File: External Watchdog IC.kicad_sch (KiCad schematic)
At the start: 10 parts, among them U4 TPS3823A-33DBVR, U5 TPS3823A-33DBVR

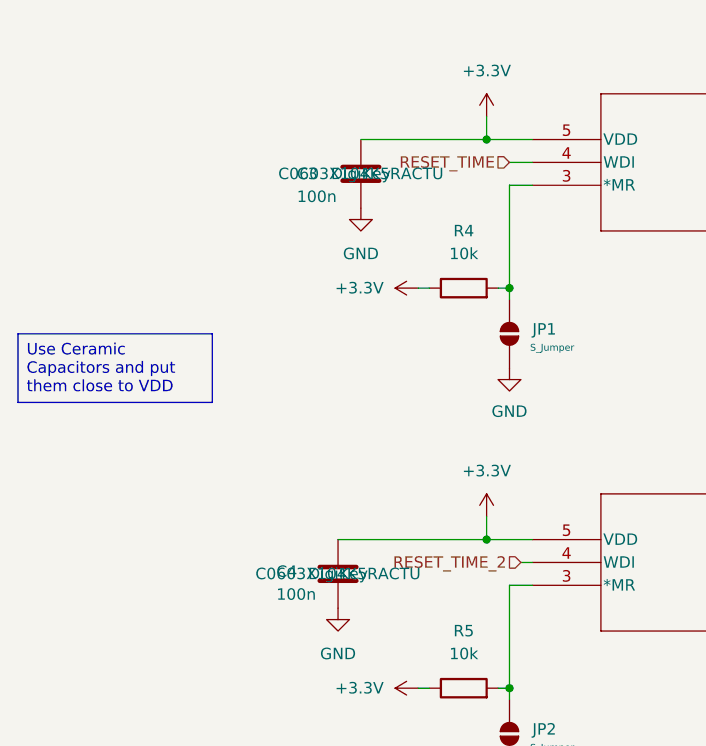
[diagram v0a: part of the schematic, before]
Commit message: Added footprints to caps
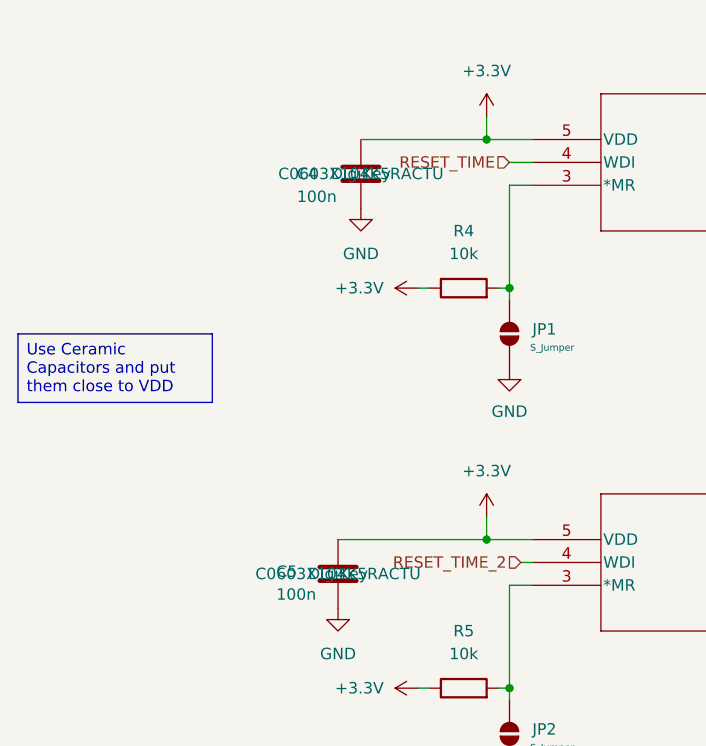
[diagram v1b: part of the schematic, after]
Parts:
- renumbered C3 to C4, C4 to C5
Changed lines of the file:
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@@
 		(on_board yes)
 		(dnp no)
-		(property "Reference" "C3"
+		(property "Reference" "C4"
 			(at 94.488 76.2 0)
 			(effects
@@
 			(project ""
 				(path "/8f246f89-1ec7-4136-9977-839b50e116ed/61eb8b07-a516-4600-8bd8-c85438ae98cc"
-					(reference "C3")
+					(reference "C4")
 					(unit 1)
 				)
@@
 		(on_board yes)
 		(dnp no)
-		(property "Reference" "C4"
+		(property "Reference" "C5"
 			(at 92.202 120.396 0)
 			(effects
@@
 			(project "EPS_mppt_board"
 				(path "/8f246f89-1ec7-4136-9977-839b50e116ed/61eb8b07-a516-4600-8bd8-c85438ae98cc"
-					(reference "C4")
-					(unit 1)
-				)
+					(reference "C5")
+					(unit 1)
+				)
